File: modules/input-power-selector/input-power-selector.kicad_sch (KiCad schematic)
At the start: 37 parts, among them Q1 SI4909DY-T1-GE3, Q2 SI4909DY-T1-GE3, Q3 SI4909DY-T1-GE3, Q4 IPF067N20NM6ATMA1, Q7 BC847, U1 LTC4417IGN, U2 SQJQ141EL-T1_GE3

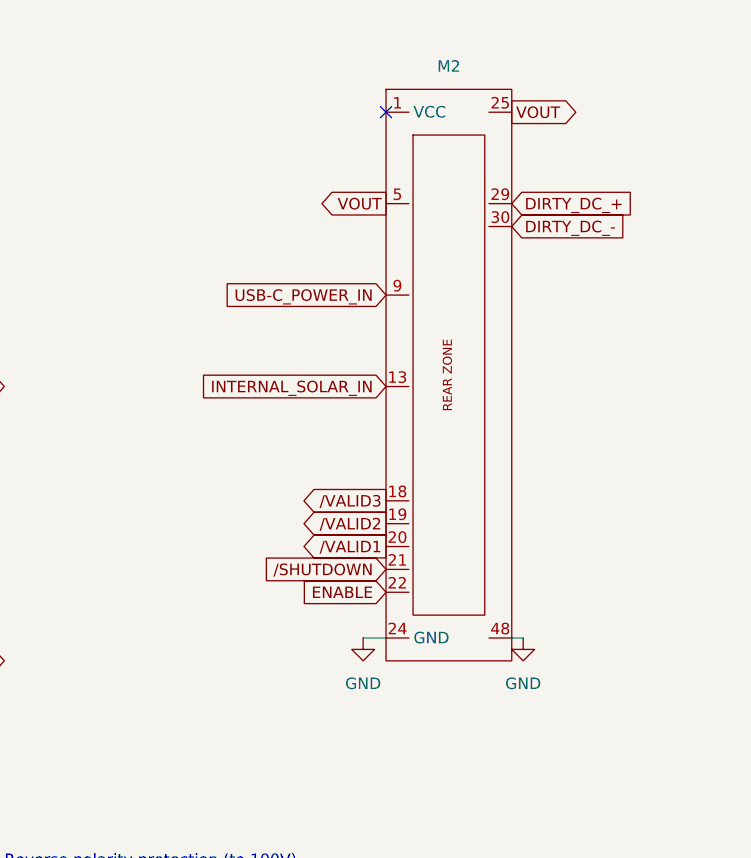
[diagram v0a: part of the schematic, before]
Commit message: Updating all modules
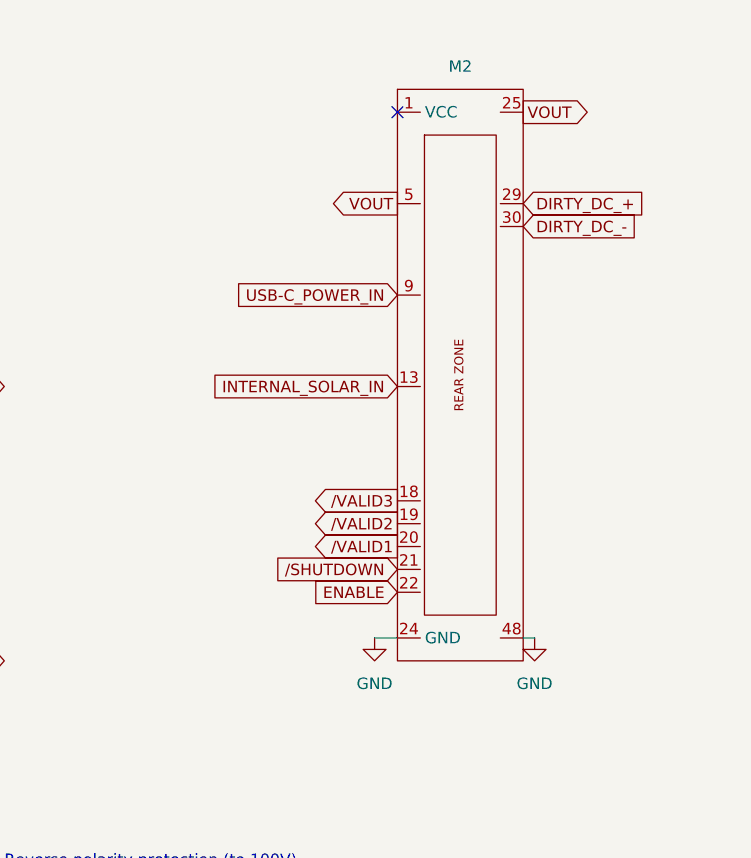
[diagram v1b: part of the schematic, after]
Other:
- moved on the sheet: M2
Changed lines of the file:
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@@
 	)
 	(no_connect
-		(at 237.49 40.64)
+		(at 238.76 40.64)
 	)
 	(wire
@@
 	(wire
 		(pts
-			(xy 251.46 99.06) (xy 252.73 99.06)
+			(xy 252.73 99.06) (xy 254 99.06)
 		)
 		(stroke
@@
 	(wire
 		(pts
-			(xy 234.95 99.06) (xy 237.49 99.06)
+			(xy 236.22 99.06) (xy 238.76 99.06)
 		)
 		(stroke
@@
 	(global_label "DIRTY_DC_+"
 		(shape input)
-		(at 251.46 50.8 0)
+		(at 252.73 50.8 0)
 		(fields_autoplaced yes)
 		(effects
@@
 		)
 		(property "Intersheetrefs" "${INTERSHEET_REFS}"
-			(at 265.6938 50.8 0)
+			(at 266.9638 50.8 0)
 			(effects
 				(font
@@
 	(global_label "ENABLE"
 		(shape input)
-		(at 237.49 93.98 180)
+		(at 238.76 93.98 180)
 		(fields_autoplaced yes)
 		(effects
@@
 		)
 		(property "Intersheetrefs" "${INTERSHEET_REFS}"
-			(at 227.4896 93.98 0)
+			(at 228.7596 93.98 0)
 			(effects
 				(font
@@
 	(global_label "{slash}VALID1"
 		(shape output)
-		(at 237.49 88.9 180)
+		(at 238.76 88.9 180)
 		(fields_autoplaced yes)
 		(effects
@@
 		)
 		(property "Intersheetrefs" "${INTERSHEET_REFS}"
-			(at 226.8847 88.9 0)
+			(at 228.1547 88.9 0)
 			(effects
 				(font
@@
 	(global_label "USB-C_POWER_IN"
 		(shape input)
-		(at 237.49 60.96 180)
+		(at 238.76 60.96 180)
 		(fields_autoplaced yes)
 		(effects
@@
 		)
 		(property "Intersheetrefs" "${INTERSHEET_REFS}"
-			(at 217.511 60.96 0)
+			(at 218.781 60.96 0)
 			(effects
 				(font
@@
 	(global_label "{slash}SHUTDOWN"
 		(shape input)
-		(at 237.49 91.44 180)
+		(at 238.76 91.44 180)
 		(fields_autoplaced yes)
 		(effects
@@
 		)
 		(property "Intersheetrefs" "${INTERSHEET_REFS}"
-			(at 222.9538 91.44 0)
+			(at 224.2238 91.44 0)
 			(effects
 				(font
@@
 	(global_label "VOUT"
 		(shape output)
-		(at 237.49 50.8 180)
+		(at 238.76 50.8 180)
 		(fields_autoplaced yes)
 		(effects
@@
 		)
 		(property "Intersheetrefs" "${INTERSHEET_REFS}"
-			(at 229.7876 50.8 0)
+			(at 231.0576 50.8 0)
 			(effects
 				(font
@@
 	(global_label "VOUT"
 		(shape output)
-		(at 251.46 40.64 0)
+		(at 252.73 40.64 0)
 		(fields_autoplaced yes)
 		(effects
@@
 		)
 		(property "Intersheetrefs" "${INTERSHEET_REFS}"
-			(at 259.1624 40.64 0)
+			(at 260.4324 40.64 0)
 			(effects
 				(font
@@
 	(global_label "{slash}VALID3"
 		(shape output)
-		(at 237.49 83.82 180)
+		(at 238.76 83.82 180)
 		(fields_autoplaced yes)
 		(effects
@@
 		)
 		(property "Intersheetrefs" "${INTERSHEET_REFS}"
-			(at 226.8847 83.82 0)
+			(at 228.1547 83.82 0)
 			(effects
 				(font
@@
 	(global_label "{slash}VALID2"
 		(shape output)
-		(at 237.49 86.36 180)
+		(at 238.76 86.36 180)
 		(fields_autoplaced yes)
 		(effects
@@
 		)
 		(property "Intersheetrefs" "${INTERSHEET_REFS}"
-			(at 226.8847 86.36 0)
+			(at 228.1547 86.36 0)
 			(effects
 				(font
@@
 	(global_label "DIRTY_DC_-"
 		(shape input)
-		(at 251.46 53.34 0)
+		(at 252.73 53.34 0)
 		(fields_autoplaced yes)
 		(effects
@@
 		)
 		(property "Intersheetrefs" "${INTERSHEET_REFS}"
-			(at 265.6938 53.34 0)
+			(at 266.9638 53.34 0)
 			(effects
 				(font
@@
 	(global_label "INTERNAL_SOLAR_IN"
 		(shape input)
-		(at 237.49 71.12 180)
+		(at 238.76 71.12 180)
 		(fields_autoplaced yes)
 		(effects
@@
 		)
 		(property "Intersheetrefs" "${INTERSHEET_REFS}"
-			(at 215.9385 71.12 0)
+			(at 217.2085 71.12 0)
 			(effects
 				(font
@@
 	(symbol
 		(lib_id "power:GND")
-		(at 252.73 99.06 0)
+		(at 254 99.06 0)
 		(unit 1)
 		(exclude_from_sim no)
@@
 		(fields_autoplaced yes)
 		(property "Reference" "#PWR20"
-			(at 252.73 105.41 0)
+			(at 254 105.41 0)
 			(effects
 				(font
@@
 		)
 		(property "Value" "GND"
-			(at 252.73 104.14 0)
+			(at 254 104.14 0)
 			(effects
 				(font
@@
 		)
 		(property "Footprint" ""
-			(at 252.73 99.06 0)
+			(at 254 99.06 0)
 			(effects
 				(font
@@
 		)
 		(property "Datasheet" ""
-			(at 252.73 99.06 0)
+			(at 254 99.06 0)
 			(effects
 				(font
@@
 		)
 		(property "Description" "Power symbol creates a global label with name \"GND\" , ground"
-			(at 252.73 99.06 0)
+			(at 254 99.06 0)
 			(effects
 				(font
@@
 	(symbol
 		(lib_id "power:GND")
-		(at 234.95 99.06 0)
+		(at 236.22 99.06 0)
 		(unit 1)
 		(exclude_from_sim no)
@@
 		(fields_autoplaced yes)
 		(property "Reference" "#PWR19"
-			(at 234.95 105.41 0)
+			(at 236.22 105.41 0)
 			(effects
 				(font
@@
 		)
 		(property "Value" "GND"
-			(at 234.95 104.14 0)
+			(at 236.22 104.14 0)
 			(effects
 				(font
@@
 		)
 		(property "Footprint" ""
-			(at 234.95 99.06 0)
+			(at 236.22 99.06 0)
 			(effects
 				(font
@@
 		)
 		(property "Datasheet" ""
-			(at 234.95 99.06 0)
+			(at 236.22 99.06 0)
 			(effects
 				(font
@@
 		)
 		(property "Description" "Power symbol creates a global label with name \"GND\" , ground"
-			(at 234.95 99.06 0)
+			(at 236.22 99.06 0)
 			(effects
 				(font
@@
 	(symbol
 		(lib_id "MegaCastle:MegaCastle2x24-Module-I42.0x56.2-M88887D8C0001")
-		(at 243.84 69.85 0)
+		(at 245.11 69.85 0)
 		(unit 1)
 		(exclude_from_sim no)
@@
 		(fields_autoplaced yes)
 		(property "Reference" "M2"
-			(at 244.475 35.56 0)
+			(at 245.745 35.56 0)
 			(effects
 				(font
@@
 		)
 		(property "Value" "~"
-			(at 244.475 36.83 0)
+			(at 245.745 36.83 0)
 			(effects
 				(font
@@
 		)
 		(property "Footprint" "MegaCastle:MegaCastle2x24-Module-I47.0x56.2-M88887D8C0001-SPAREPAD"
-			(at 243.84 106.68 0)
+			(at 245.11 106.68 0)
 			(effects
 				(font
@@
 		)
 		(property "Datasheet" ""
-			(at 243.84 64.77 0)
+			(at 245.11 64.77 0)
 			(effects
 				(font
@@
 		)
 		(property "Description" "Generated using footprint-gen .. 42 55 14 M88887D8C0001"
-			(at 243.84 69.85 0)
+			(at 245.11 69.85 0)
 			(effects
 				(font
